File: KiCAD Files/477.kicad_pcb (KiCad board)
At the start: 2 copper layers, 101.7 x 59.6 mm, 85 parts, among them IC1 W25N01GVSFIG, IC2 W25N01GVSFIG, IC3 W25N01GVSFIG, IC4 W25N01GVSFIG, IC5 AZ1117IH-3.3TRG1, IC6 USBLC6-2SC6, J1 BM06B-SRSS-TBT_LF__SN_, J2 6364372-2, J3 TSW-103-14-S-D, J4 TSW-103-14-S-D, J5 BM07B-SRSS-TB_LF__SN_, J6 BM09B-SRSS-TB_LF__SN_, J7 TSW-105-05-F-S, U1 STM32H7A3RGTx, Y1 ABM8G-48.000MHZ-18-D2Y-T

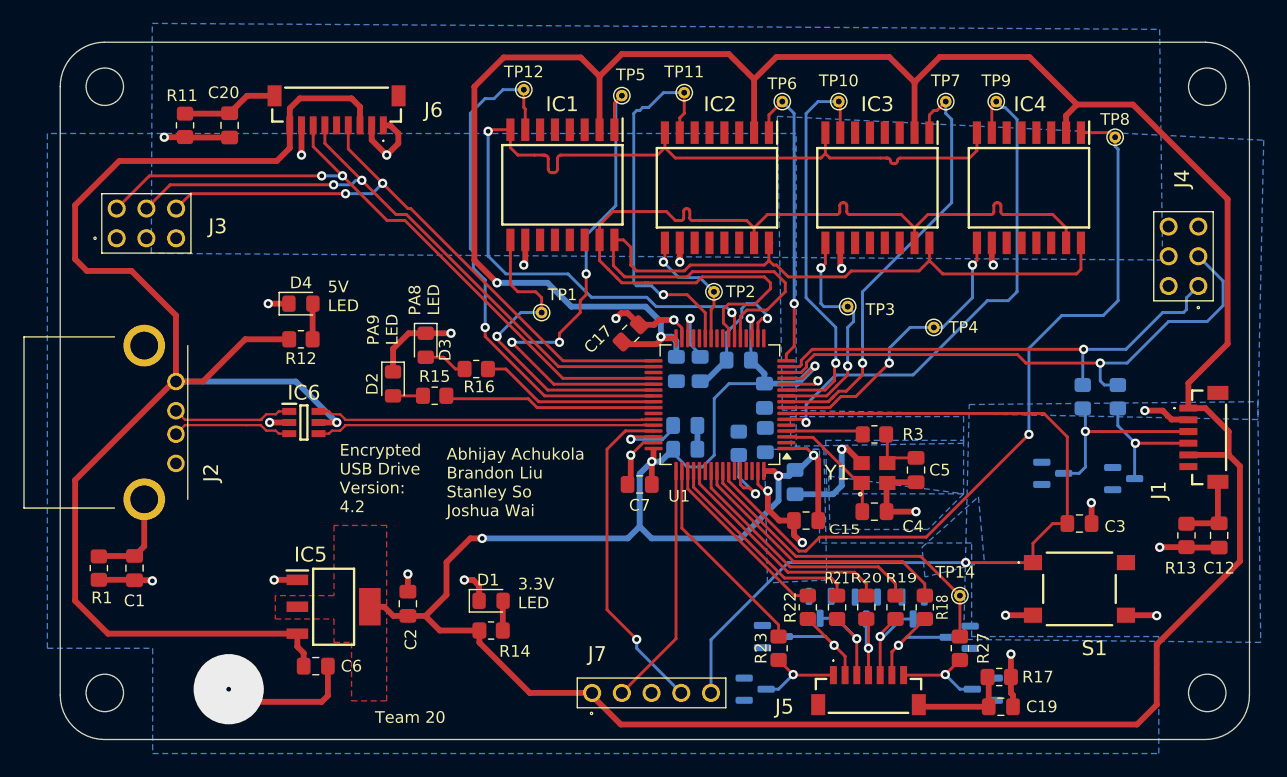
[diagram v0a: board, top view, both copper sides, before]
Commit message: made a few tweaks based on setsuna's comments
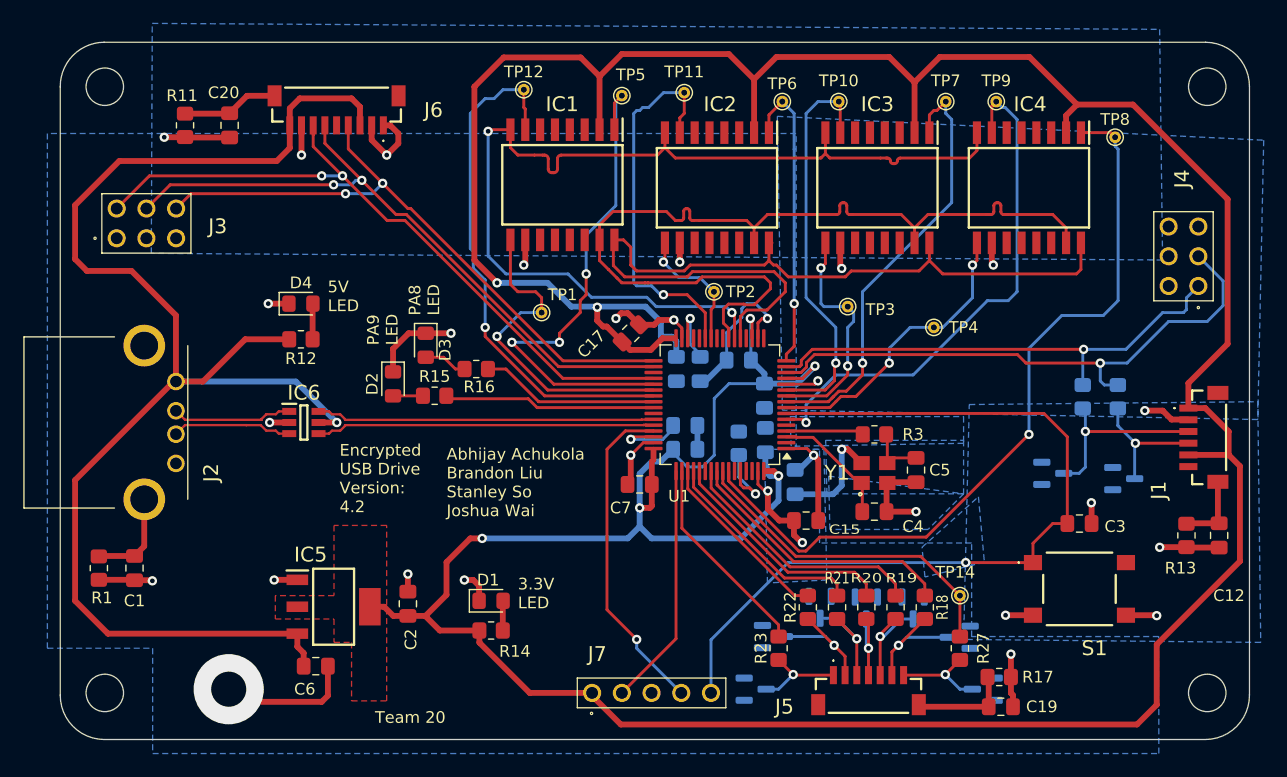
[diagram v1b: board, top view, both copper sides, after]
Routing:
- net VBAT: track 354.3 -> 362.8 mm
- net PA1/FP RX ESD: track 43.0 -> 42.3 mm
- net unconnected-(J4-Pad2): track 0.70 -> 0.00 mm
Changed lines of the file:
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@@
 		(tags "capacitor handsolder")
 		(property "Reference" "C7"
-			(at 0 -1.778 0)
+			(at 1.628 -2 0)
 			(layer "F.SilkS")
 			(effects
@@
 		(tags "capacitor handsolder")
 		(property "Reference" "C17"
-			(at -2.334867 -1.616446 45)
+			(at -3.027831 -1.732412 45)
 			(layer "F.SilkS")
 			(effects
@@
 		(tags "capacitor handsolder")
 		(property "Reference" "C6"
-			(at 3.048 0 0)
+			(at -0.942 1.968 0)
 			(layer "F.SilkS")
 			(effects
@@
 		(tags "capacitor handsolder")
 		(property "Reference" "C12"
-			(at 2.794 0 180)
+			(at 5.144 -0.842 180)
 			(layer "F.SilkS")
 			(effects
@@
 		)
 		(property "Value" "BZX84Cxx"
-			(at 0 -2.4 360)
+			(at 0 -2.4 0)
 			(layer "B.Fab")
 			(hide yes)
@@
 		)
 		(property "Footprint" "Package_TO_SOT_SMD:SOT-23"
-			(at 0 0 360)
+			(at 0 0 0)
 			(layer "B.Fab")
 			(hide yes)
@@
 		)
 		(property "Datasheet" "https://diotec.com/tl_files/diotec/files/pdf/datasheets/bzx84c2v4.pdf"
-			(at 0 0 360)
+			(at 0 0 0)
 			(layer "B.Fab")
 			(hide yes)
@@
 		)
 		(property "Description" "300mW Zener Diode, SOT-23"
-			(at 0 0 360)
+			(at 0 0 0)
 			(layer "B.Fab")
 			(hide yes)
@@
 		(tags "SOT TO_SOT_SMD")
 		(property "Reference" "D11"
-			(at 0 2.682 360)
+			(at 0 2.682 0)
 			(layer "B.SilkS")
 			(effects
@@
 		)
 		(property "Value" "BZX84Cxx"
-			(at 0 -2.4 360)
+			(at 0 -2.4 0)
 			(layer "B.Fab")
 			(hide yes)
@@
 		)
 		(property "Footprint" "Package_TO_SOT_SMD:SOT-23"
-			(at 0 0 360)
+			(at 0 0 0)
 			(layer "B.Fab")
 			(hide yes)
@@
 		)
 		(property "Datasheet" "https://diotec.com/tl_files/diotec/files/pdf/datasheets/bzx84c2v4.pdf"
-			(at 0 0 360)
+			(at 0 0 0)
 			(layer "B.Fab")
 			(hide yes)
@@
 		)
 		(property "Description" "300mW Zener Diode, SOT-23"
-			(at 0 0 360)
+			(at 0 0 0)
 			(layer "B.Fab")
 			(hide yes)
@@
 		)
 		(property "Value" "BZX84Cxx"
-			(at 0 -2.4 360)
+			(at 0 -2.4 0)
 			(layer "B.Fab")
 			(hide yes)
@@
 		)
 		(property "Footprint" "Package_TO_SOT_SMD:SOT-23"
-			(at 0 0 360)
+			(at 0 0 0)
 			(layer "B.Fab")
 			(hide yes)
@@
 		)
 		(property "Datasheet" "https://diotec.com/tl_files/diotec/files/pdf/datasheets/bzx84c2v4.pdf"
-			(at 0 0 360)
+			(at 0 0 0)
 			(layer "B.Fab")
 			(hide yes)
@@
 		)
 		(property "Description" "300mW Zener Diode, SOT-23"
-			(at 0 0 360)
+			(at 0 0 0)
 			(layer "B.Fab")
 			(hide yes)
@@
 		(at 100 131)
 		(size 6)
-		(drill 0.4)
+		(drill 3)
 		(layers "F.Cu" "B.Cu")
 		(free yes)
@@
 	)
 	(segment
+		(start 136 115.5)
+		(end 135.128 115.5)
+		(width 0.5)
+		(layer "F.Cu")
+		(net 57)
+	)
+	(segment
 		(start 172.514 81.026)
 		(end 177.292 81.026)
@@
 	)
 	(segment
+		(start 136.1655 113.5)
+		(end 136.1655 115.3345)
+		(width 0.5)
+		(layer "F.Cu")
+		(net 57)
+	)
+	(segment
 		(start 130.086 77)
 		(end 131.699 78.613)
@@
 	)
 	(segment
+		(start 132.314754 100)
+		(end 132 100)
+		(width 0.5)
+		(layer "F.Cu")
+		(net 57)
+	)
+	(segment
 		(start 136.1655 111.5445)
 		(end 136.1655 113.5)
@@
 	)
 	(segment
+		(start 132 100)
+		(end 131.5 99.5)
+		(width 0.5)
+		(layer "F.Cu")
+		(net 57)
+	)
+	(segment
 		(start 131.699 78.613)
 		(end 131.699 83.174)
@@
 	)
 	(segment
+		(start 131.5 99.5)
+		(end 131.5 98.35)
+		(width 0.5)
+		(layer "F.Cu")
+		(net 57)
+	)
+	(segment
 		(start 168.45 76.962)
 		(end 160.782 76.962)
@@
 	)
 	(segment
-		(start 137.073 101.005)
-		(end 136.578 101.5)
+		(start 121 94.33)
+		(end 121 79.5)
 		(width 0.5)
 		(layer "F.Cu")
@@
 	)
 	(segment
-		(start 133.814754 101.5)
-		(end 133.632377 101.317623)
+		(start 118.043 125.984)
+		(end 121.428 125.984)
 		(width 0.5)
 		(layer "F.Cu")
@@
 	)
 	(segment
-		(start 121 94.33)
-		(end 121 79.5)
+		(start 137.073 101.005)
+		(end 136.078 102)
 		(width 0.5)
 		(layer "F.Cu")
@@
 	)
 	(segment
-		(start 118.043 125.984)
-		(end 121.428 125.984)
+		(start 185.383 101.487)
+		(end 185.383 89.117)
 		(width 0.5)
 		(layer "F.Cu")
@@
 	)
 	(segment
-		(start 185.383 101.487)
-		(end 185.383 89.117)
+		(start 134.314754 102)
+		(end 133.632377 101.317623)
 		(width 0.5)
 		(layer "F.Cu")
@@
 	)
 	(segment
-		(start 136.578 101.5)
-		(end 133.814754 101.5)
+		(start 136.078 102)
+		(end 134.314754 102)
 		(width 0.5)
 		(layer "F.Cu")
@@
 	)
 	(segment
-		(start 137.073 101.005)
-		(end 136.93825 100.87025)
-		(width 0.25)
+		(start 136.1655 115.3345)
+		(end 136 115.5)
+		(width 0.5)
 		(layer "F.Cu")
 		(net 57)
@@
 	)
 	(segment
+		(start 133.632377 101.317623)
+		(end 132.314754 100)
+		(width 0.5)
+		(layer "F.Cu")
+		(net 57)
+	)
+	(segment
 		(start 121.428 125.984)
 		(end 121.428 127.016)
@@
 	)
 	(via
-		(at 136.1655 111.5445)
+		(at 135.128 115.5)
 		(size 0.8)
 		(drill 0.4)
@@
 	)
 	(via
-		(at 136.93825 100.87025)
+		(at 131.5 98.35)
 		(size 0.8)
 		(drill 0.4)
@@
 	)
 	(segment
+		(start 147 112.765)
+		(end 146.265 112.765)
+		(width 0.5)
+		(layer "B.Cu")
+		(net 57)
+	)
+	(segment
 		(start 141.5 111)
 		(end 141.5 106.15)
@@
 	)
 	(segment
+		(start 146 112.5)
+		(end 146 112)
+		(width 0.5)
+		(layer "B.Cu")
+		(net 57)
+	)
+	(segment
 		(start 137.9875 110.8095)
 		(end 139.178 112)
@@
 	)
 	(segment
-		(start 147 112.765)
-		(end 147.906 112.765)
+		(start 135.128 112.582)
+		(end 136.1655 111.5445)
 		(width 0.5)
 		(layer "B.Cu")
@@
 	)
 	(segment
-		(start 135.128 112.582)
-		(end 136.1655 111.5445)
-		(width 0.5)
+		(start 146 112)
+		(end 145.8685 111.8685)
+		(width 0.25)
 		(layer "B.Cu")
 		(net 57)
@@
 	)
 	(segment
-		(start 147.906 112.765)
-		(end 148.411 112.26)
-		(width 0.5)
-		(layer "B.Cu")
-		(net 57)
-	)
-	(segment
 		(start 121.666 118.11)
 		(end 134.112 118.11)
@@
 	)
 	(segment
+		(start 146.265 112.765)
+		(end 146 112.5)
+		(width 0.5)
+		(layer "B.Cu")
+		(net 57)
+	)
+	(segment
 		(start 129.286 98.298)
 		(end 135.636 98.298)
@@
 	)
 	(segment
+		(start 145.8685 111.8685)
+		(end 145.8685 110.744)
+		(width 0.5)
+		(layer "B.Cu")
+		(net 57)
+	)
+	(segment
 		(start 144.6345 99.3625)
 		(end 144.586 99.314)
@@
 	)
 	(segment
-		(start 179.846 97.028)
-		(end 180.34 96.534)
-		(width 0.25)
-		(layer "F.Cu")
-		(net 105)
-	)
-	(segment
 		(start 155.686 126.5)
 		(end 155.686 126.314)
@@
 	)
 	(segment
-		(start 183.388 97.042)
-		(end 182.88 96.534)
-		(width 0.25)
-		(layer "F.Cu")
-		(net 126)
-	)
-	(segment
